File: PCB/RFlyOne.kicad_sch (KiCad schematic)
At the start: 168 parts, among them J1 UFL, J2 UFL, Q1 AO3401A, Q2 AO3401A, SW1 TS24CA, SW2 TS24CA, SW4 TS24CA, SW5 TS24CA, U1 TQP3M9036, U10 ATGM332D-5N31, U11 ESP32_S3_MINI, U12 E80-900M2212S, U13 RT9193-33GB, U14 RT8097CHGE, U15 BMI270, U16 MMC5983MA, U17 BQ25606RGER, U18 TPS61023DRLR, U19 CH32V003F4U6, U2 TLV3201, U20 TXU0202DTTR, U21 TPS7A0230-3V0, U22 240x320_2.4in_TFT, U3 TA0970A, U4 TQP3M9036, U5 TA0970A, U6 AD8313ARMZ, U7 RP2040, U8 W25Q128, U9 12MHz

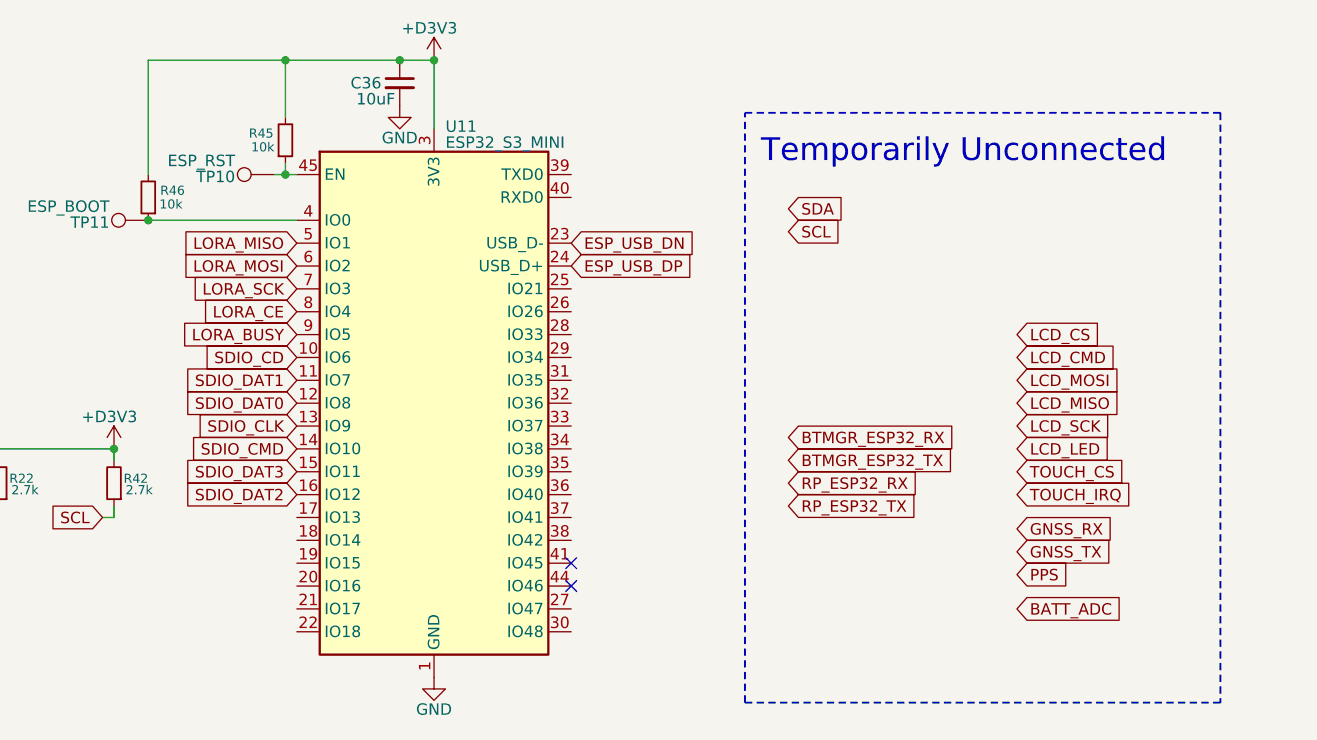
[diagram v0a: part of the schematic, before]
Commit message: checkpoint
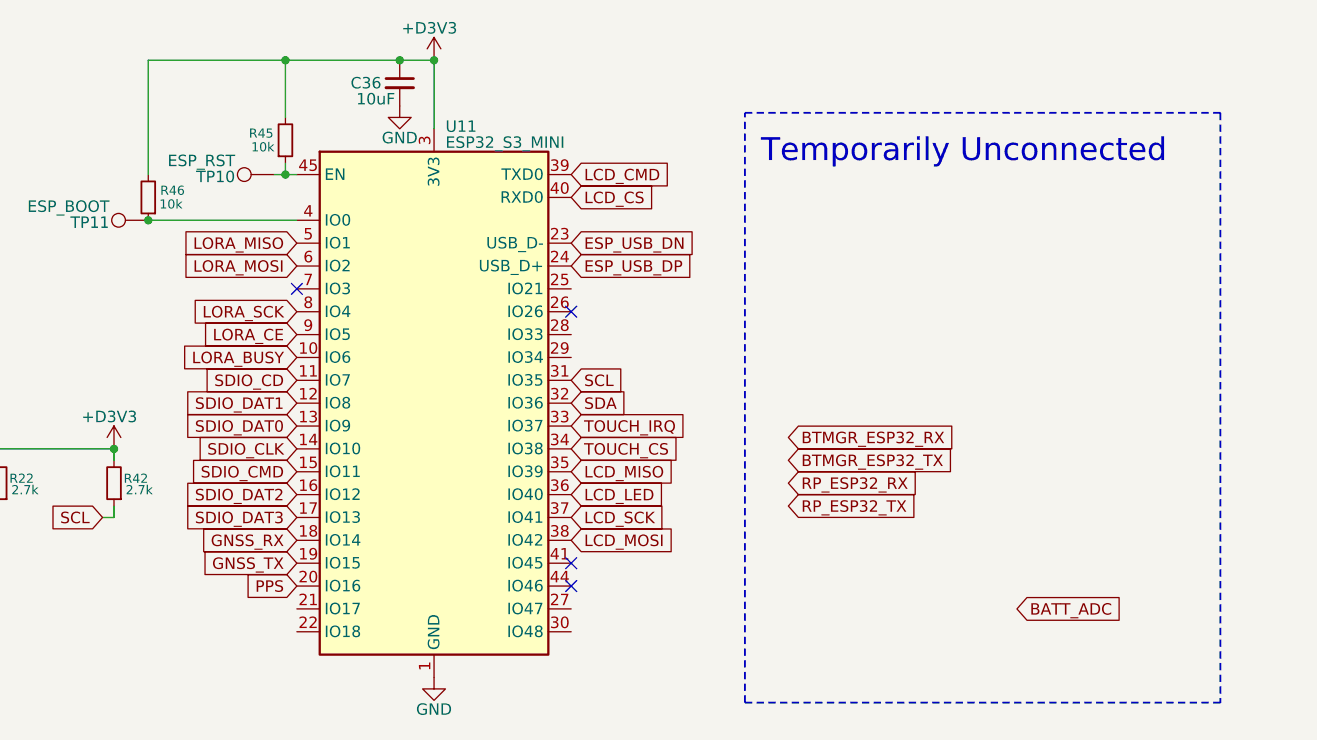
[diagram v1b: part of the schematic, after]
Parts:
- L5, L6, L7: footprint Inductor_SMD:L_Changjiang_FTC201610S -> easyeda2kicad:L_Changjiang_FTC201610S
- TP1, TP10, TP11, TP2, TP3, TP4, TP5, TP6, TP7, TP8, TP9: footprint (none) -> easyeda2kicad:TestPoint
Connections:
- net GNSS_RX: now also U11.18 (IO14)
- net GNSS_TX: now also U11.19 (IO15)
- net LCD_CMD: now also U11.39 (TXD0)
- net LCD_CS: now also U11.40 (RXD0)
- net LCD_LED: now also U11.36 (IO40)
- net LCD_MISO: now also U11.35 (IO39)
- net LCD_MOSI: now also U11.38 (IO42)
- net LCD_SCK: now also U11.37 (IO41)
- net LORA_BUSY: now also U11.10 (IO6); no longer U11.9 (IO5)
- net LORA_CE: now also U11.9 (IO5); no longer U11.8 (IO4)
- net LORA_SCK: now also U11.8 (IO4); no longer U11.7 (IO3)
- net PPS: now also U11.20 (IO16)
- net SCL: now also U11.31 (IO35)
- net SDA: now also U11.32 (IO36)
- net SDIO_CD: now also U11.11 (IO7); no longer U11.10 (IO6)
- net SDIO_CLK: now also U11.14 (IO10); no longer U11.13 (IO9)
- net SDIO_CMD: now also U11.15 (IO11); no longer U11.14 (IO10)
- net SDIO_DAT0: now also U11.13 (IO9); no longer U11.12 (IO8)
- net SDIO_DAT1: now also U11.12 (IO8); no longer U11.11 (IO7)
- net SDIO_DAT3: now also U11.17 (IO13); no longer U11.15 (IO11)
- net TOUCH_CS: now also U11.34 (IO38)
- net TOUCH_IRQ: now also U11.33 (IO37)
- no-connect marks 80 -> 82
